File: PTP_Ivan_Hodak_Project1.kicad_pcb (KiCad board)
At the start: 2 copper layers, 42 parts, among them SW1 SW_Push, SW2 SW_SPDT, U0 NE555P, U1 LM2574N-5, U2 4027, U3 4027, U4 74LS47

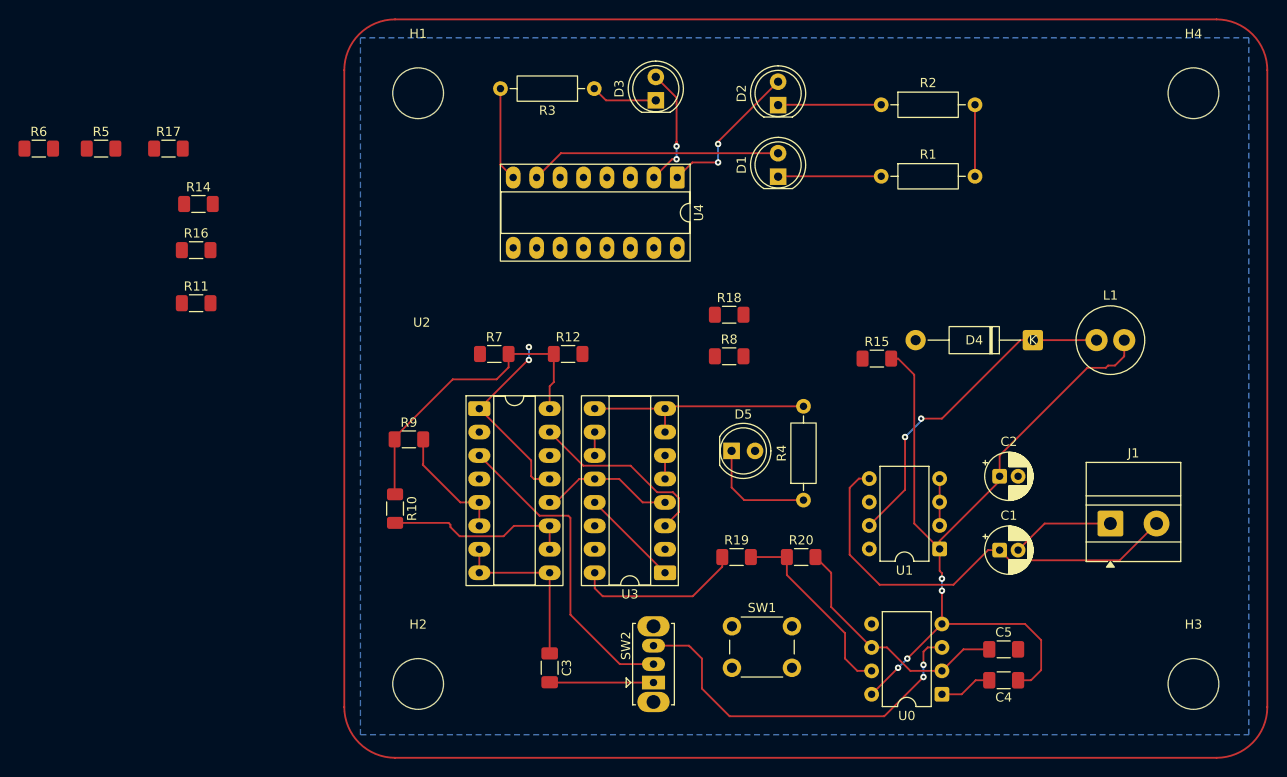
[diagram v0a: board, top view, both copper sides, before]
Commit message: Update projekta
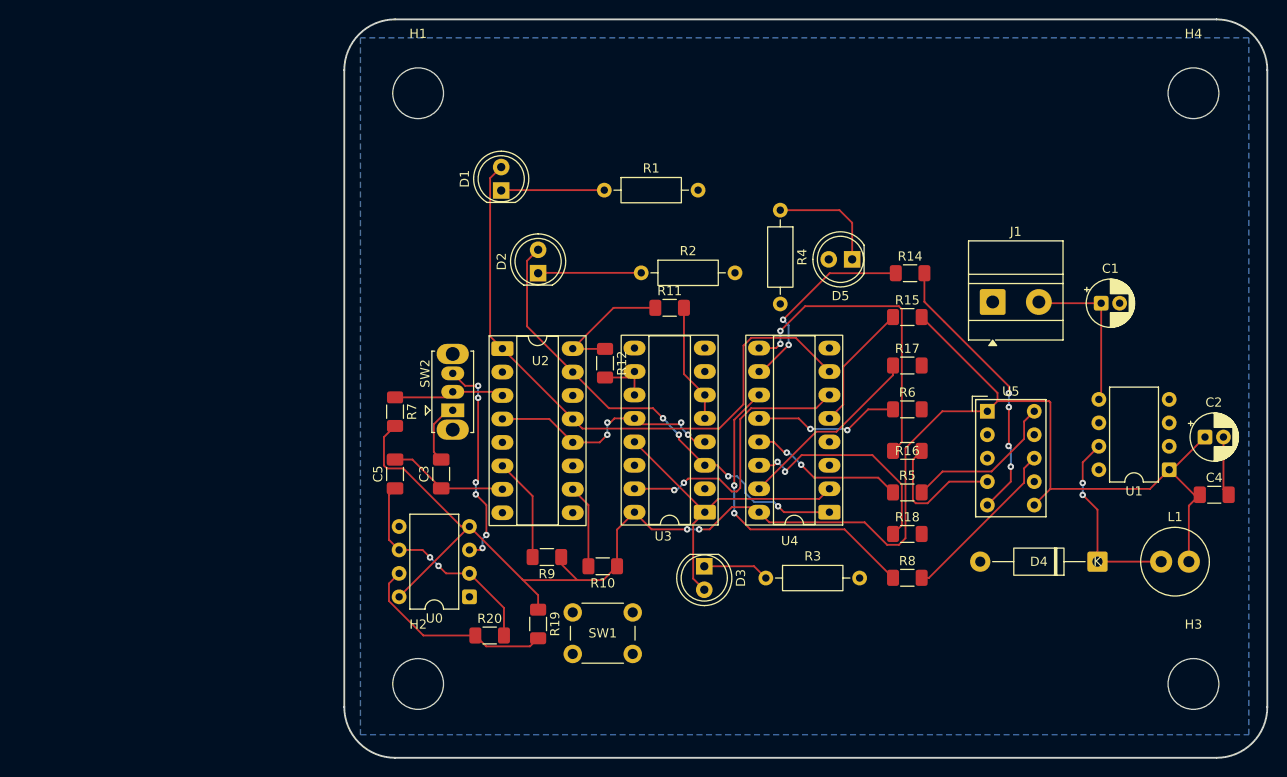
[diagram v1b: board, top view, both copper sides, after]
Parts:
- added U5: FYS-3911BUHR-21, Display_7Segment:HDSP-7401, F.Cu at (175.7, 102.5)
- moved R6 98.2 mm to (167.0, 102.2)
- moved R5 95.0 mm to (167.0, 111.2)
- moved R17 83.4 mm to (167.0, 97.5)
- moved R16 80.1 mm to (167.0, 106.8)
- moved R14 77.5 mm to (167.3, 87.5)
- moved C5 68.6 mm to (111.5, 109.2), turned to 90 degrees
- moved R3 56.2 mm to (151.7, 120.5), turned to 0 degrees
- moved U0 52.3 mm to (119.6, 122.6)
- moved R11 51.3 mm to (141.2, 91.2)
- moved D3 50.7 mm to (145.0, 119.2), turned to -90 degrees
- moved U4 39.8 mm to (158.6, 113.4), turned to 180 degrees
- moved SW2 36.7 mm to (117.8, 102.3)
- moved R20 34.8 mm to (121.8, 126.8)
- moved D2 31.7 mm to (127.0, 87.5)
- moved R2 31.7 mm to (138.2, 87.5)
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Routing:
- net GND: track 84.1 -> 19.4 mm
- net +5V: track 144.8 -> 191.1 mm, vias 4 -> 2
- net Net-(U4-e): track 0.00 -> 34.0 mm, vias 0 -> 2
- net Net-(U4-c): track 0.00 -> 34.0 mm, vias 0 -> 2
- net Q3: track 0.00 -> 31.0 mm, vias 0 -> 2
- net VD: track 48.0 -> 17.3 mm
- net Net-(U5-D): track 0.00 -> 30.1 mm, vias 0 -> 4
- net Net-(U4-g): track 0.00 -> 24.0 mm, vias 0 -> 2
- net Clock: track 34.4 -> 12.0 mm
- net Net-(U4-d): track 0.00 -> 21.7 mm, vias 0 -> 2
- net Q0: track 48.0 -> 69.0 mm, vias 2 -> 0
- net Net-(U4-f): track 0.00 -> 20.7 mm
- net Net-(U5-C): track 0.00 -> 18.5 mm
- net 555: track 41.0 -> 23.1 mm, vias 2 -> 6
- net Net-(U5-A): track 0.00 -> 17.0 mm
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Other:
- board outline added: 100 x 80 mm
